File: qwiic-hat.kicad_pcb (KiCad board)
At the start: 2 copper layers, 16.2 x 72 mm, 6 parts, among them J1 Conn_02x20_Odd_Even, J2 Conn_01x04_Male, J3 Conn_01x04_Male, J4 Conn_01x03_Pin

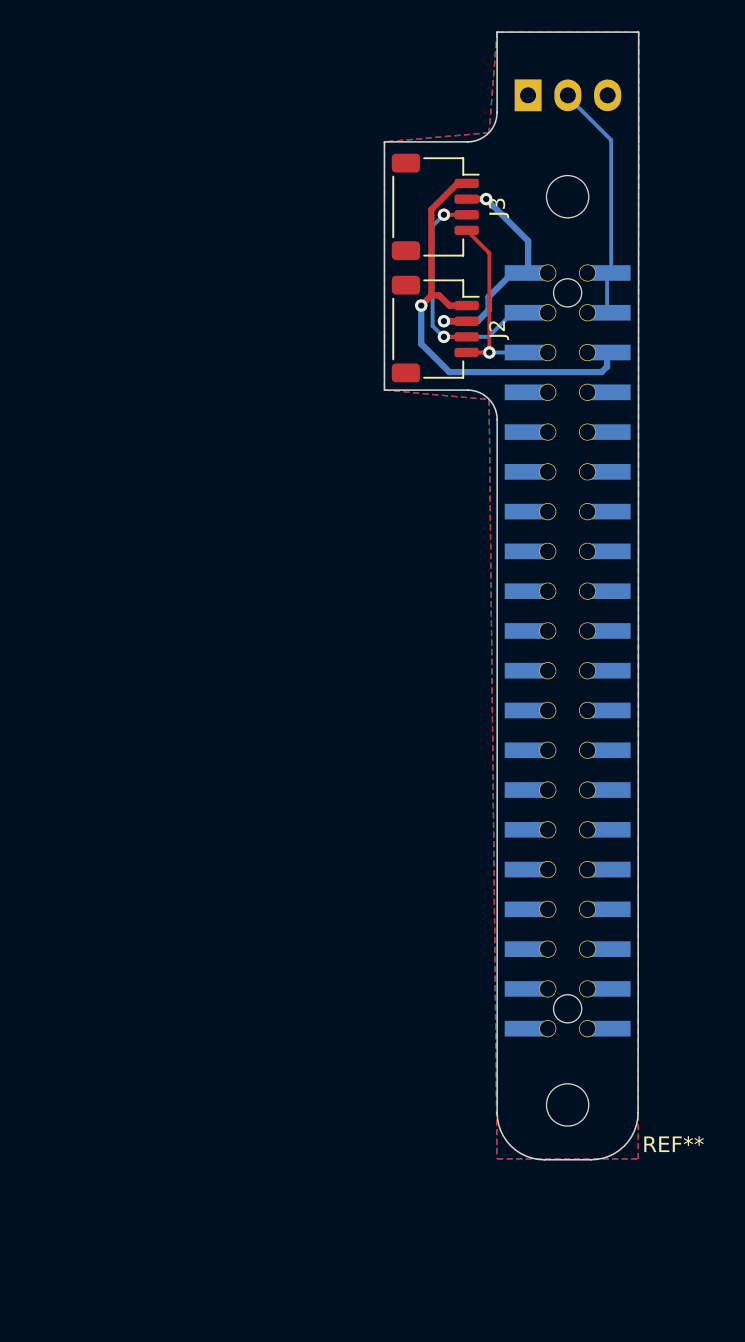
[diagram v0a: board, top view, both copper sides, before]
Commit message: cleanup sheets
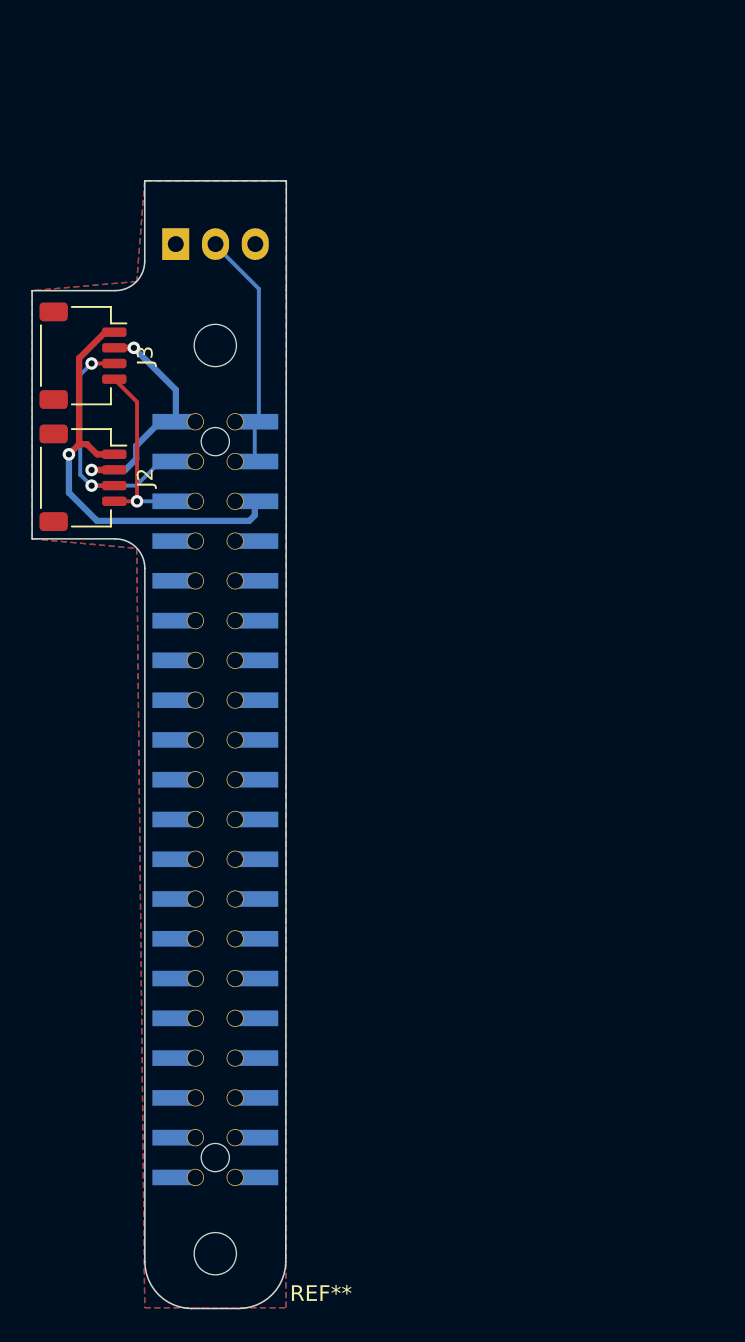
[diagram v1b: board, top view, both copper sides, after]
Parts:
- moved J4 24.4 mm to (150.5, 73.0)
- moved J1 24.4 mm to (153.0, 108.5)
- moved J2 24.4 mm to (144.6, 88.0)
- moved J3 24.4 mm to (144.6, 80.2)
- moved REF** 24.4 mm to (153.0, 137.5)
- moved REF** 24.4 mm to (153.0, 79.5)
